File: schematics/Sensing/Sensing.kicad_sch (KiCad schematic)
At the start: 16 parts, among them J1 Conn_01x02_Pin, J2 Conn_01x05_Pin, J3 Conn_01x05_Pin, SW1 SW_SPST, SW2 SW_Push, U2 TCS34725FN, U3 ESP32C3_Xiao

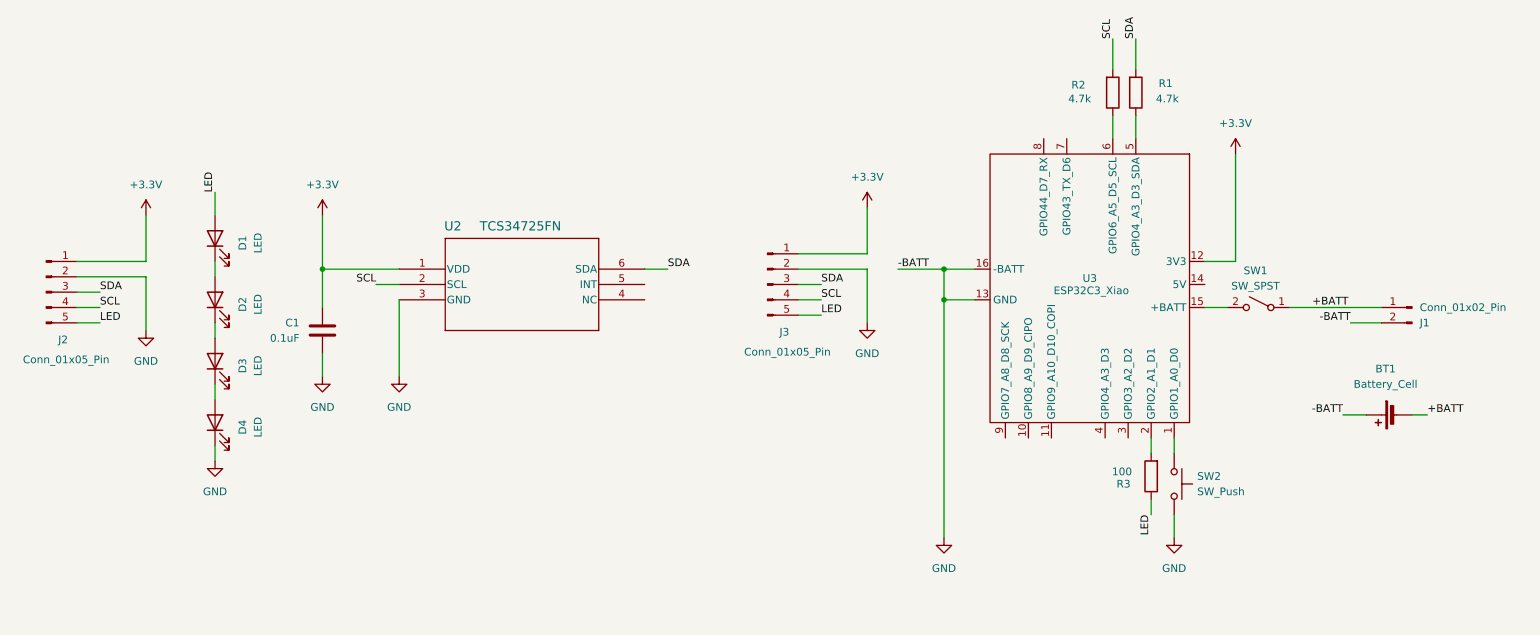
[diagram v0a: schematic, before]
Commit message: Update PCB and Enclosure Designs
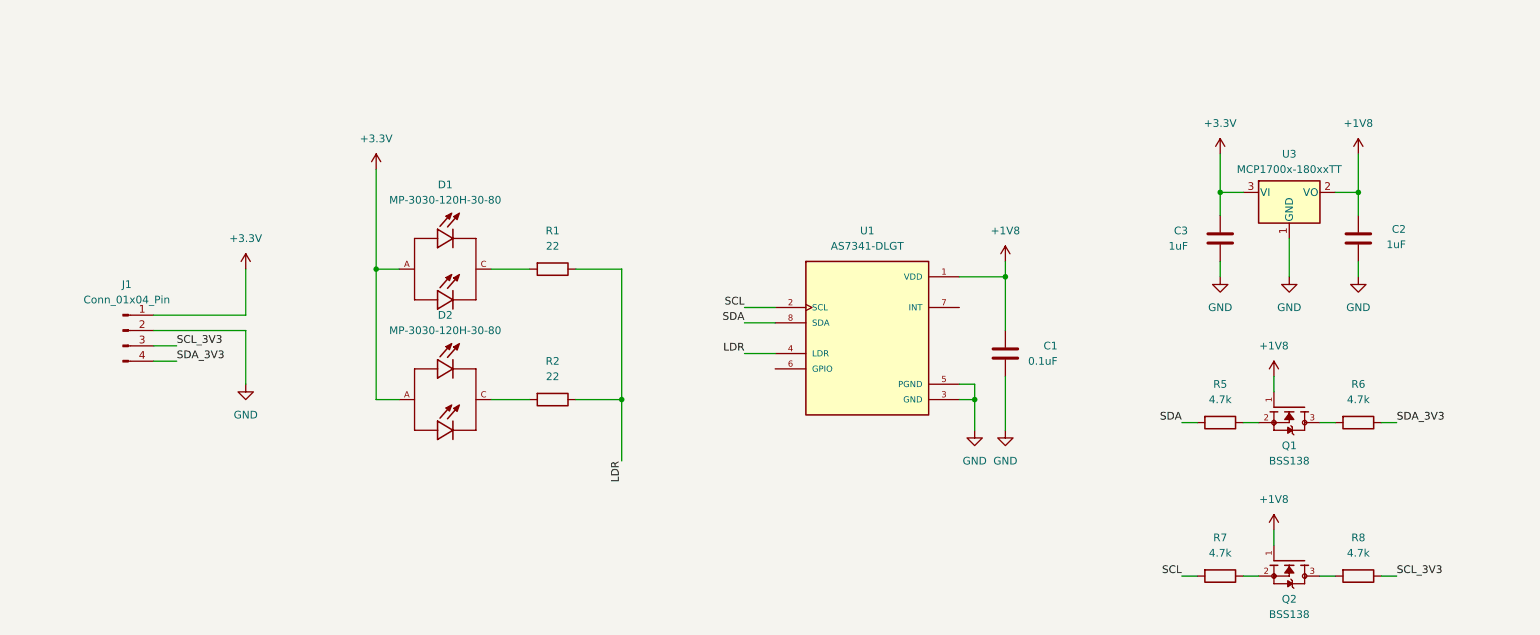
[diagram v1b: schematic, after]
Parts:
- removed BT1: Battery_Cell, Xiao_Seeed_ESP32C3:MOUDLE14P-SMD-2.54-21X17.8MM, symbol Device:Battery_Cell
- removed D1, D2, D3, D4: LED, LED_SMD:LED_0603_1608Metric_Pad1.05x0.95mm_HandSolder, symbol Device:LED
- removed J1: Conn_01x02_Pin, Connector_PinSocket_2.54mm:PinSocket_1x02_P2.54mm_Vertical, symbol Connector:Conn_01x02_Pin
- removed J2, J3: Conn_01x05_Pin, Connector_PinSocket_2.54mm:PinSocket_1x05_P2.54mm_Vertical, symbol Connector:Conn_01x05_Pin
- removed R3: 100, Resistor_SMD:R_0603_1608Metric_Pad0.98x0.95mm_HandSolder, symbol Device:R
- removed SW1: SW_SPST, Button_Switch_SMD:SW_SPST_EVQPE1, symbol Switch:SW_SPST
- removed SW2: SW_Push, Button_Switch_SMD:SW_SPDT_PCM12, symbol Switch:SW_Push
- removed U2: TCS34725FN, TCS34725:TCS34725FN_AMS, symbol 2026-01-26_22-08-00:TCS34725FN
- removed U3: ESP32C3_Xiao, ESP32_Xiao_Seeed_GIX:XIAO_ESP32, symbol sensorcircuits:XIAO_ESP32
- added C2, C3: 1uF, Capacitor_SMD:C_0603_1608Metric_Pad1.08x0.95mm_HandSolder, symbol Device:C
- added D1, D2: MP-3030-120H-30-80, MP_3030_120H_30_80:LED_MP-3030-120H-30-80, symbol sensorcircuits:MP-3030-120H-30-80
- added J1: Conn_01x04_Pin, Connector_PinSocket_2.54mm:PinSocket_1x04_P2.54mm_Vertical, symbol Connector:Conn_01x04_Pin
- added Q1, Q2: BSS138, BSS138:SOT-23_3L_ONS, symbol sensorcircuits:BSS138
- added R5, R6, R7, R8: 4.7k, Resistor_SMD:R_0603_1608Metric_Pad0.98x0.95mm_HandSolder, symbol Device:R
- added U1: AS7341-DLGT, AS7341_DLGT:SON8_AS7341-DLGM_AMS, symbol sensorcircuits:AS7341-DLGT
- added U3: MCP1700x-180xxTT, Package_TO_SOT_SMD:SOT-23, symbol Regulator_Linear:MCP1700x-180xxTT
- R1, R2: value 4.7k -> 22
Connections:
- net +3.3V: now also C3.1, D1.A, D2.A, J1.1 (Pin_1), U3.3 (VI); no longer C1.1
- net GND: now also C2.2, C3.2, J1.2 (Pin_2), U1.3 (GND), U1.5 (PGND), U3.1 (GND)
- net SCL: now also R7.2, U1.2 (SCL); no longer R2.2
- net SDA: now also R5.2, U1.8 (SDA); no longer R1.2
- net LDR: now reaches R1.1
- net LDR: now also R2.1, U1.4 (LDR)
- new net: D1.C, R1.2
- new net: Q1.3, R6.2
- new net: Q1.2, R5.1
- new net: Q2.3, R8.2
- new net: Q2.2, R7.1
- new net: D2.C, R2.2
- new net +1V8: C1.1, C2.1, Q1.1, Q2.1, U1.1 (VDD), U3.2 (VO)
- new net SCL_3V3: J1.3 (Pin_3), R8.1
- new net SDA_3V3: J1.4 (Pin_4), R6.1
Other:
- title: Sensing Device (Pen) -> Sensing Device (Pen) - Sensor Tip
- moved on the sheet: C1
